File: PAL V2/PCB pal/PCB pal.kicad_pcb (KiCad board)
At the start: 2 copper layers, 35.2 x 83.7 mm, 8 parts, among them J1 Conn_01x04_MountingPin, J2 Conn_01x02, M1 Motor_Servo, M2 Motor_Servo, M3 Motor_Servo, M4 Motor_Servo, P1 USB_C_Plug_USB2.0, U1 ESP32-C6-DEVKITC-1-N8

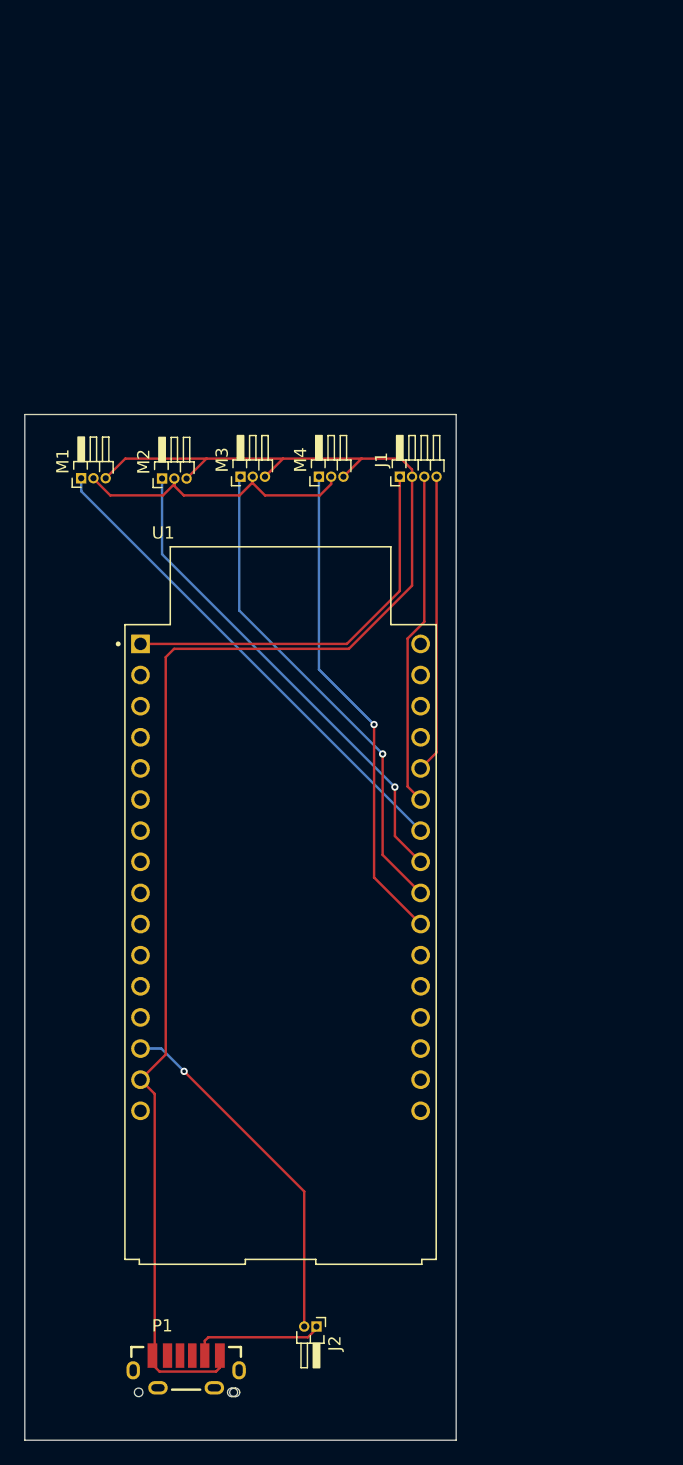
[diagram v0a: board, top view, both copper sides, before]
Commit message: New PCB changes
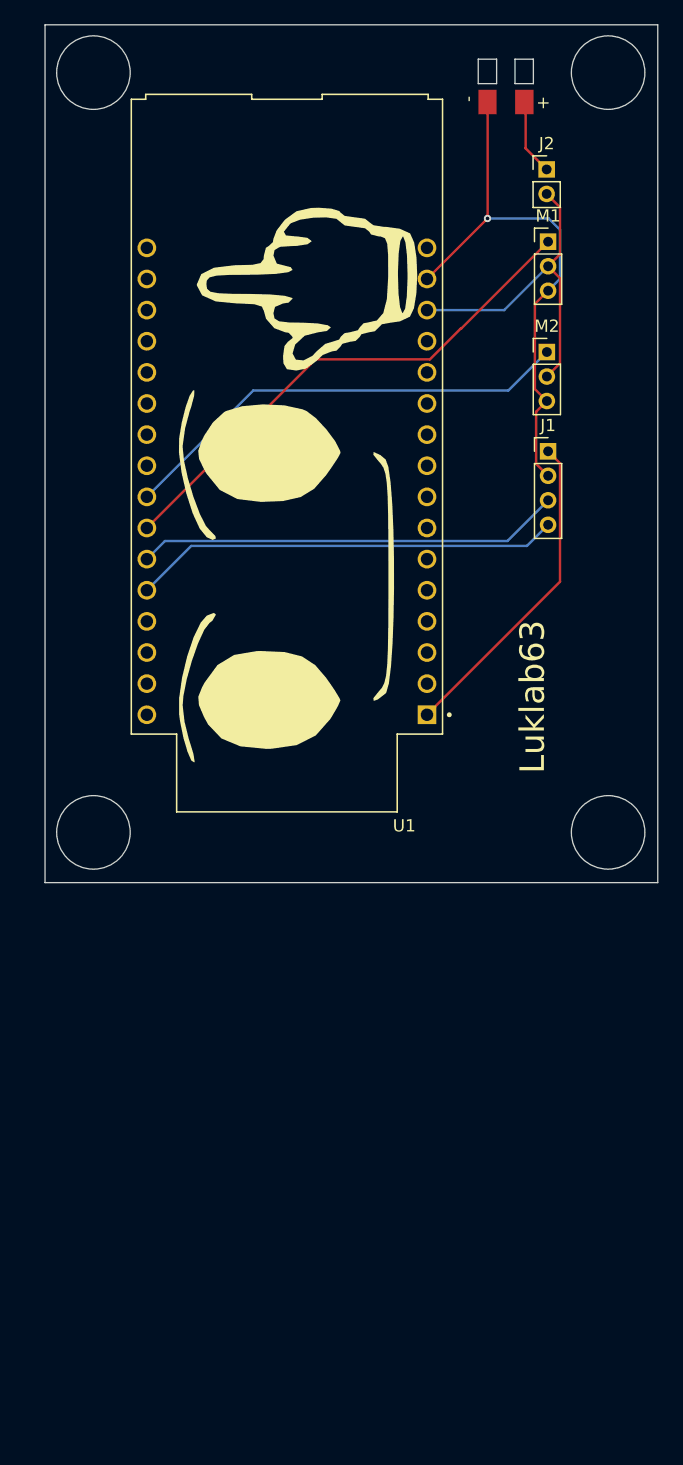
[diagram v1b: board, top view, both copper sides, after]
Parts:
- removed M3, M4: Motor_Servo, Connector_PinHeader_1.00mm:PinHeader_1x03_P1.00mm_Horizontal
- removed P1: USB_C_Plug_USB2.0, USBC:GCT_USB4140-GF-0070-C_REVA3
- added ?: LOGO, faces:fuck, F.Cu at (33.8, 49.3)
- added G***: LOGO, faces:fuck, B.Cu at (31.2, 51.5)
- added J3: Conn_01x02, modified:BatteryTERMINAL, F.Cu at (49.7, 18.4)
- J1: footprint Connector_PinHeader_1.00mm:PinHeader_1x04_P1.00mm_Horizontal -> Connector_PinHeader_2.00mm:PinHeader_1x04_P2.00mm_Vertical
- J2: footprint Connector_PinHeader_1.00mm:PinHeader_1x02_P1.00mm_Horizontal -> Connector_PinHeader_2.00mm:PinHeader_1x02_P2.00mm_Vertical
- M1, M2: footprint Connector_PinHeader_1.00mm:PinHeader_1x03_P1.00mm_Horizontal -> Connector_PinHeader_2.00mm:PinHeader_1x03_P2.00mm_Vertical
- moved J2 96.3 mm to (53.0, 23.9), turned to 0 degrees
- moved U1 42.9 mm to (31.8, 44.1), turned to 180 degrees
- moved M1 42.7 mm to (53.1, 29.8), turned to 0 degrees
- moved M2 33.1 mm to (53.0, 38.8), turned to 0 degrees
- moved J1 12.3 mm to (53.1, 46.9), turned to 0 degrees
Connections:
- U1 pad J3_10: /SERVO4 -> unconnected-(U1-GPIO18-PadJ3_10)
- U1 pad J3_9: /SERVO3 -> unconnected-(U1-GPIO19-PadJ3_9)
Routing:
- net GND: track 130.5 -> 44.1 mm, vias 0 -> 1
- net /SERVO3: track 40.1 -> 0.00 mm, vias 1 -> 0
- net /SERVO4: track 39.9 -> 0.00 mm, vias 1 -> 0
- net +5V: track 53.8 -> 28.0 mm, vias 1 -> 0
- net /SDA: track 24.3 -> 35.0 mm
- net /SCL: track 27.3 -> 34.7 mm
- net +3.3V: track 32.3 -> 26.4 mm
- net Net-(J2-Pin_1): track 10.7 -> 6.26 mm
- net /SERVO2: track 40.0 -> 37.5 mm, vias 1 -> 0
- net /SERVO1: track 40.2 -> 42.4 mm
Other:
- board size 35.2 x 83.7 mm -> 50 x 70 mm
- board text added: "Luklab63"

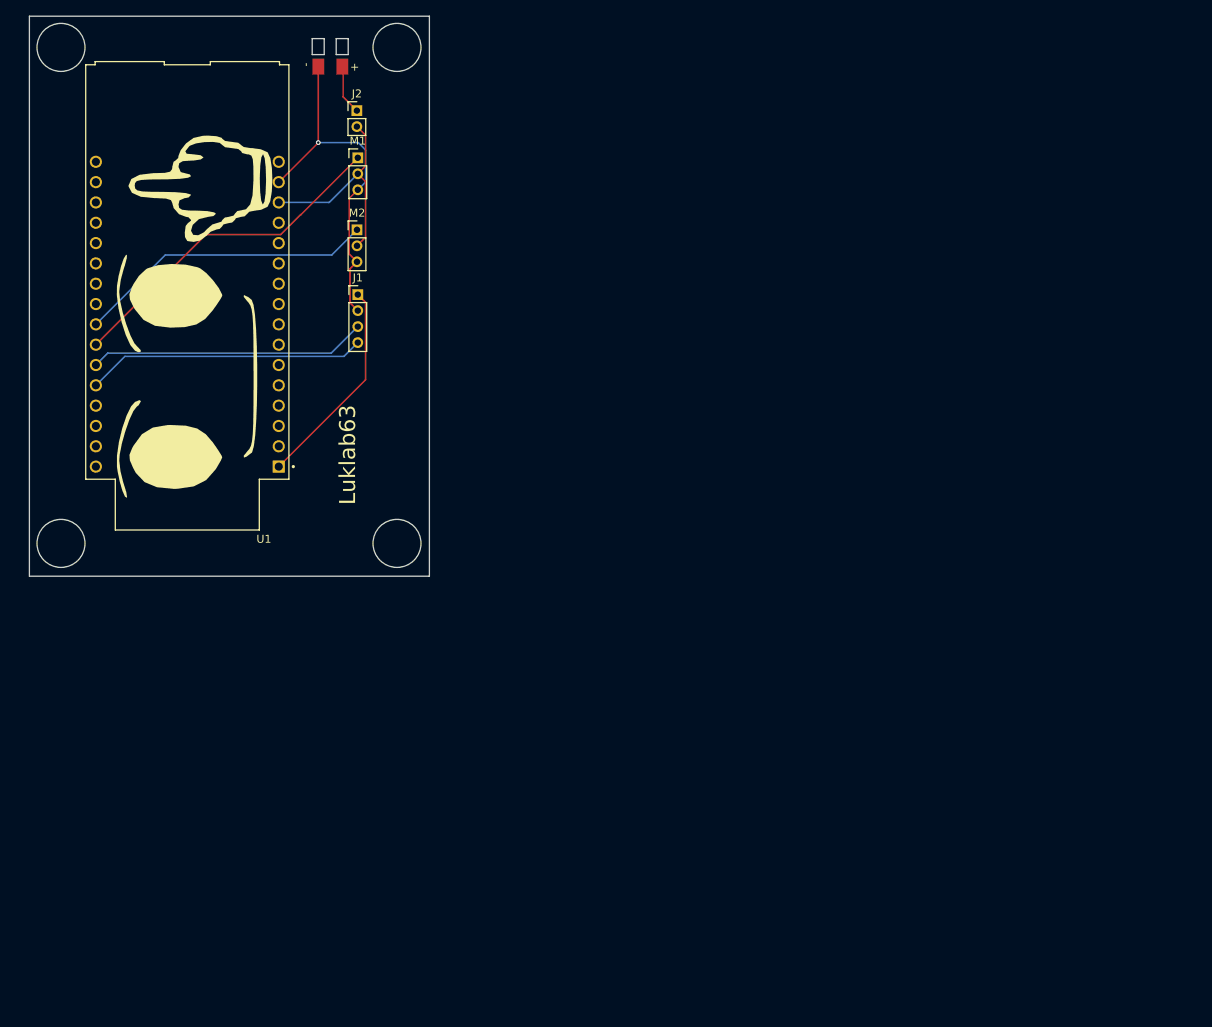
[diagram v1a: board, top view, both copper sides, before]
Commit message: shoulder mount
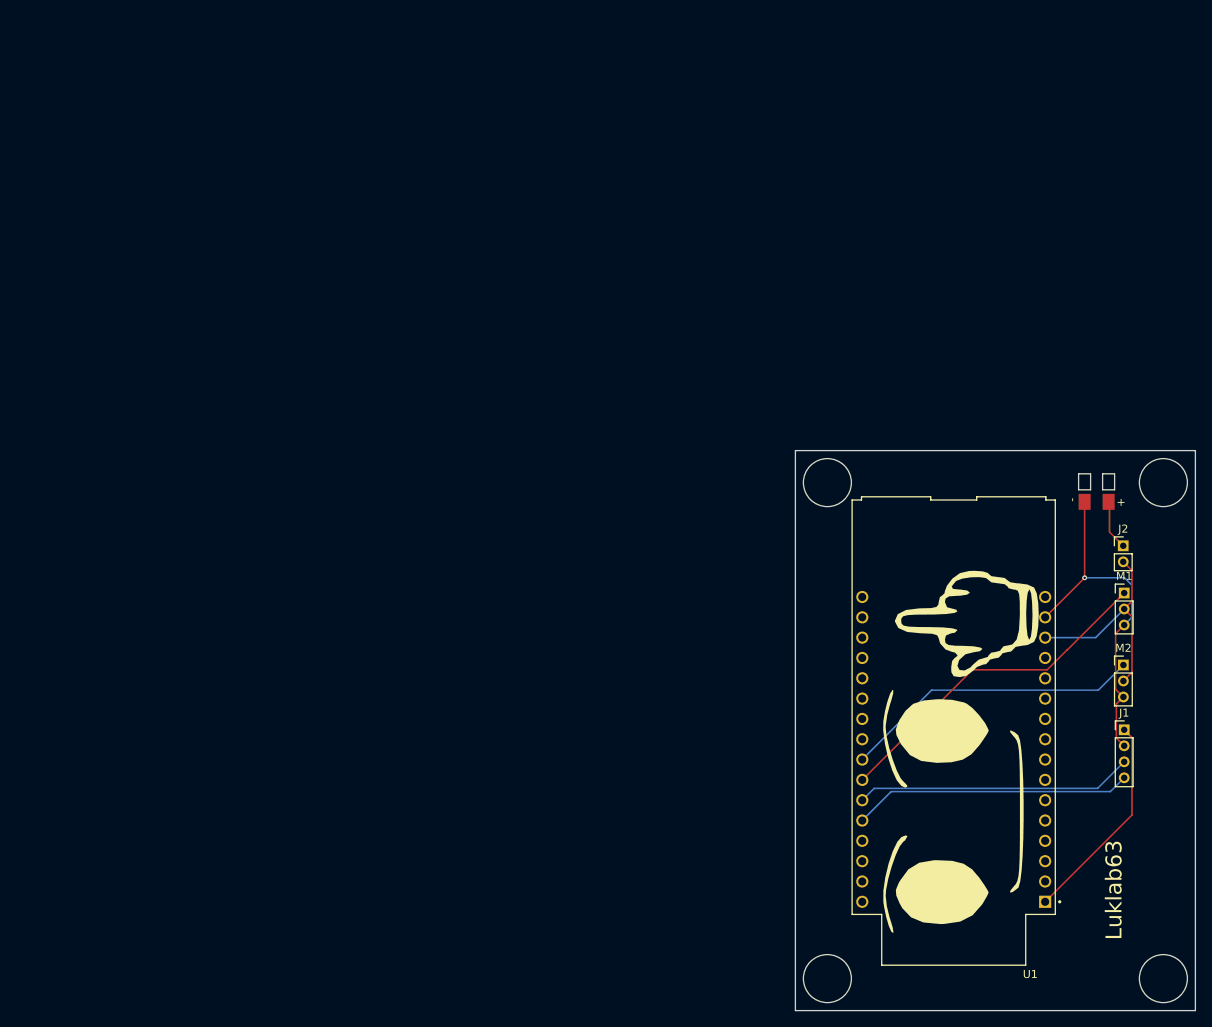
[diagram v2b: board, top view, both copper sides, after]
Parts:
- moved J1 110.2 mm to (148.9, 101.3)
- moved J3 110.2 mm to (145.5, 72.8)
- moved M1 110.2 mm to (148.9, 84.2)
- moved M2 110.2 mm to (148.8, 93.2)
- moved ? 110.2 mm to (129.6, 103.7)
- moved G*** 110.2 mm to (127.0, 105.9)
- moved U1 110.2 mm to (127.6, 98.5)
- moved J2 110.2 mm to (148.8, 78.3)
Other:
- outline, holes or cut-outs redrawn
